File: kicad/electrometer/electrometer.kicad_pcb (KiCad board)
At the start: 2 copper layers, 44.5 x 43.2 mm, 19 parts, among them J1 Screw_Terminal_01x04, J2 Screw_Terminal_01x02, J3 Conn_01x03_Male, J4 Conn_01x03_Male, M1 CD4051B, U1 LMC6082

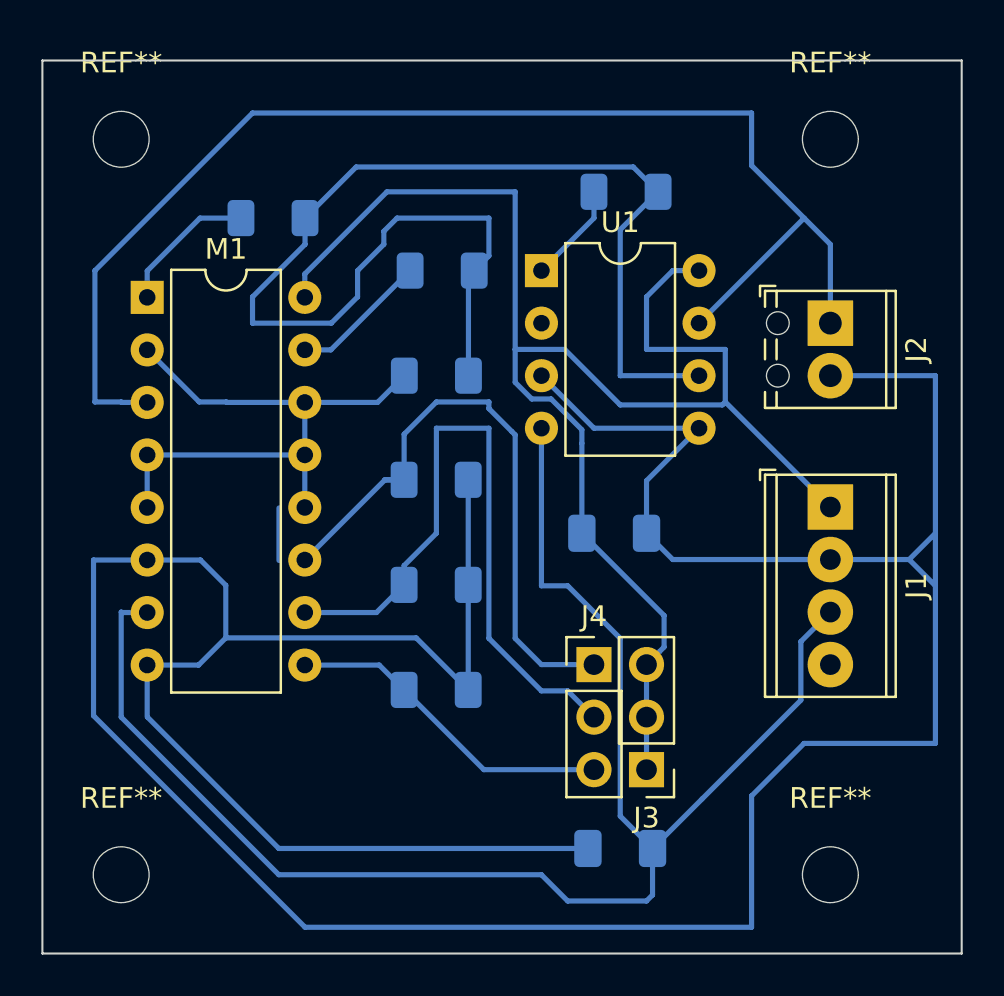
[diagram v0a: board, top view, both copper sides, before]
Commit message: updated board
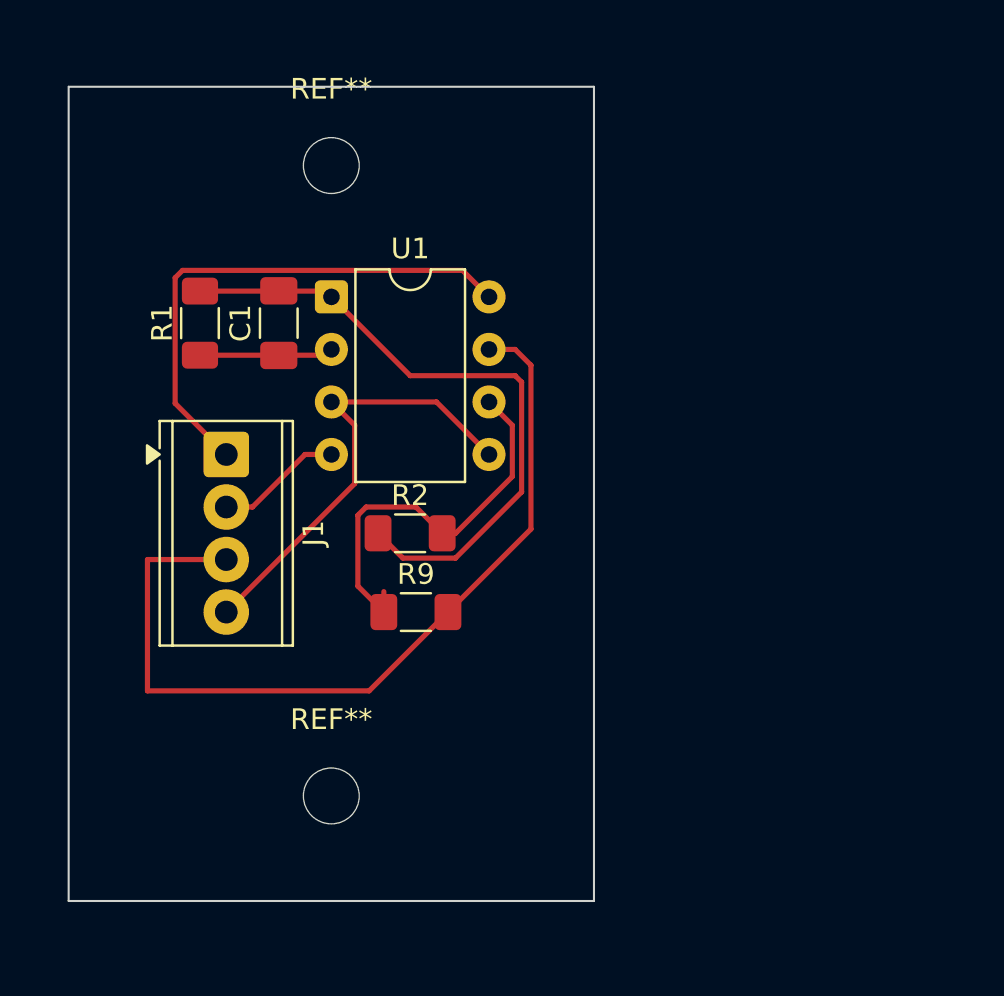
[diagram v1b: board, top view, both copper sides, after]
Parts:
- removed C2, C3: 1e-03, Capacitor_SMD:C_1206_3216Metric_Pad1.33x1.80mm_HandSolder
- removed J2: Screw_Terminal_01x02, TerminalBlock_Phoenix:TerminalBlock_Phoenix_MPT-0,5-2-2.54_1x02_P2.54mm_Horizontal
- removed J3, J4: Conn_01x03_Male, Connector_PinHeader_2.54mm:PinHeader_1x03_P2.54mm_Vertical
- removed M1: CD4051B, Package_DIP:DIP-16_W7.62mm
- removed R3: 100e+03, Resistor_SMD:R_1206_3216Metric_Pad1.30x1.75mm_HandSolder
- removed R4, R6, R7, R8: 10e+03, Resistor_SMD:R_1206_3216Metric_Pad1.30x1.75mm_HandSolder
- removed R5: 1e+03, Resistor_SMD:R_1206_3216Metric_Pad1.30x1.75mm_HandSolder
- removed the REF** at (177.8, 74.9)
- removed the REF** at (177.8, 110.5)
- added C1: 1e-03, Capacitor_SMD:C_1206_3216Metric_Pad1.33x1.80mm_HandSolder, F.Cu at (151.1, 83.8)
- added R1: 1e+03, Resistor_SMD:R_1206_3216Metric_Pad1.30x1.75mm_HandSolder, F.Cu at (147.3, 83.8)
- added R9: 1e+03, Resistor_SMD:R_1206_3216Metric_Pad1.30x1.75mm_HandSolder, F.Cu at (157.8, 97.8)
- R2: moved to F.Cu
- moved J1 29.3 mm to (148.6, 90.2)
- moved R2 19.5 mm to (157.5, 94.0)
- moved REF** 10.9 mm to (153.7, 106.7)
- moved REF** 10.2 mm to (153.7, 76.2)
- moved U1 10.2 mm to (153.7, 82.5)
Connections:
- net Net-(C2-Pad1) renamed +9V
- J1 pad 2: GND -> -9V
- J1 pad 3: Net-(C3-Pad2) -> Net-(J1-Pin_3)
- J1 pad 4: unconnected-(J1-Pad4) -> GND
- U1 pad 2: unconnected-(U1-Pad2) -> Net-(U1A--)
- U1 pad 4: Net-(C3-Pad2) -> -9V
- U1 pad 7: Net-(U1-Pad7) -> Net-(J1-Pin_3)
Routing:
- net GND: track 177.5 -> 21.9 mm
- net Net-(C3-Pad2): track 76.4 -> 0.00 mm
- net Net-(U1-Pad7): track 62.7 -> 0.00 mm
- net +9V: track 75.2 -> 25.4 mm
- net Net-(J1-Pin_3): track 0.00 -> 42.2 mm
- net Net-(U1B--): track 60.9 -> 19.6 mm
- net Net-(M1-Pad10): track 32.9 -> 0.00 mm
- net Net-(R5-Pad1): track 31.8 -> 0.00 mm
- net Net-(M1-Pad11): track 30.6 -> 0.00 mm
- net Net-(C1-Pad2): track 4.86 -> 31.5 mm
- net Net-(M1-Pad9): track 16.1 -> 0.00 mm
- net Net-(R3-Pad1): track 6.87 -> 0.00 mm
- net Net-(R4-Pad1): track 6.68 -> 0.00 mm
- net Net-(U1A--): track 0.00 -> 6.47 mm
- net -9V: track 0.00 -> 6.14 mm
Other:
- board size 44.5 x 43.2 mm -> 25.4 x 39.4 mm
